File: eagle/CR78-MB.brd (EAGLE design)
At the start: 100 x 80 mm, 44 parts, among them IC1 40106N, Q510 2N3904, Q518 2N3904, Q526 2N3904, Q7 2N3904

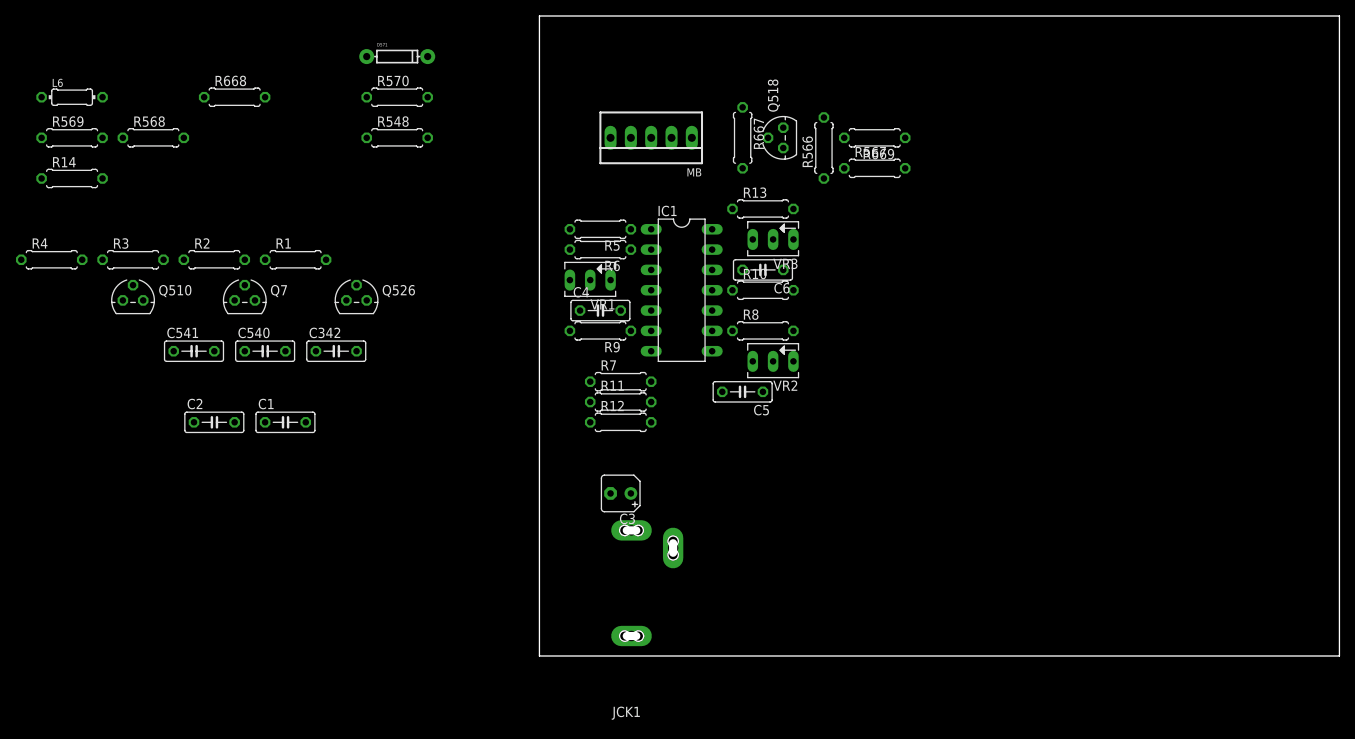
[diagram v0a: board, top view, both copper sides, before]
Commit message: parts on the brd
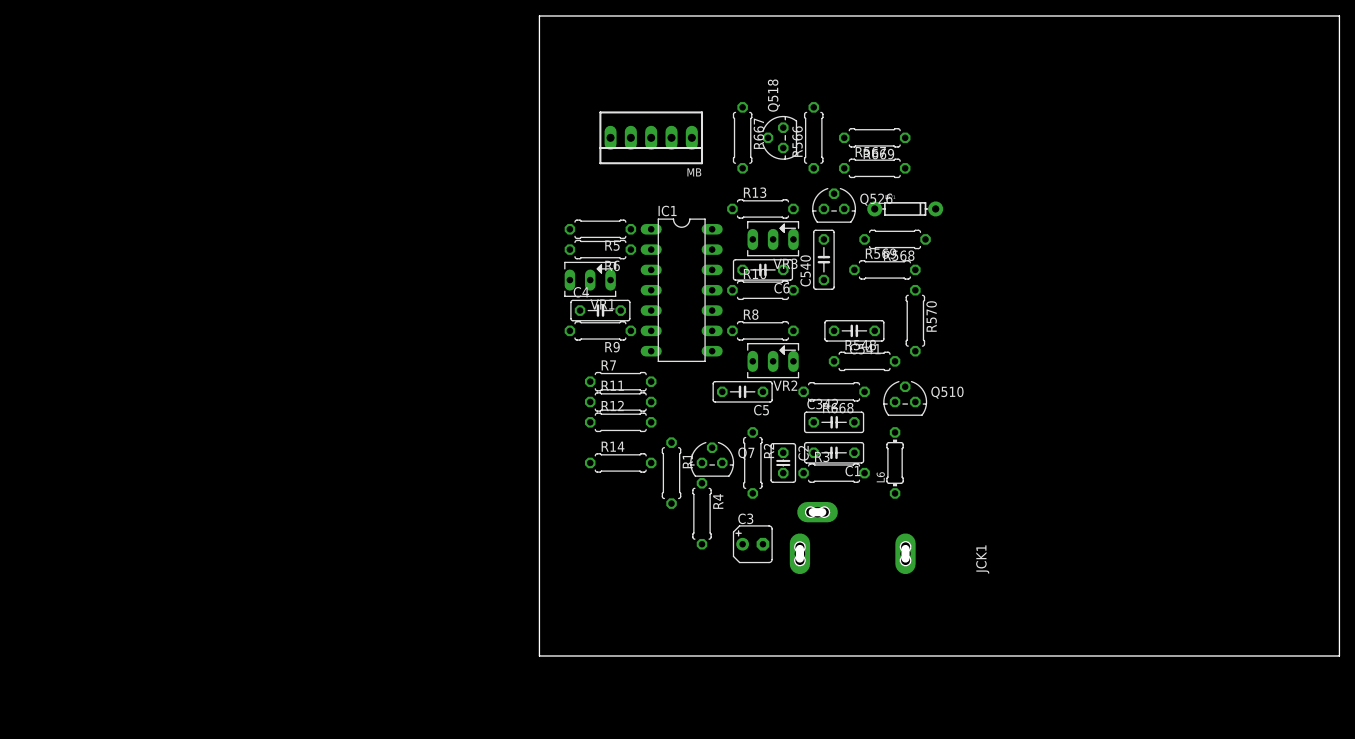
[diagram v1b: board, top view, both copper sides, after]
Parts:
- C2: device rcl:C050-025X075 -> rcl:C025-030X050
- moved L6 112.6 mm to (44.5, 24.1), turned to 90 degrees
- moved R569 102.9 mm to (43.2, 48.3)
- moved Q510 97.4 mm to (45.7, 31.8)
- moved R568 93.6 mm to (44.5, 52.1), turned to 180 degrees
- moved R3 91.6 mm to (36.8, 22.9)
- moved R4 87.3 mm to (20.3, 17.8), turned to 270 degrees
- moved R668 83.5 mm to (36.8, 33.0), turned to 180 degrees
- moved C541 82.6 mm to (39.4, 40.6), turned to 180 degrees
- moved R14 77.3 mm to (10.2, 24.1)
- moved R2 71.9 mm to (26.7, 24.1), turned to 270 degrees
- moved C2 71.3 mm to (30.5, 24.1), turned to 270 degrees
- moved C540 70.8 mm to (35.6, 49.5), turned to 90 degrees
- moved R570 70.5 mm to (47.0, 41.9), turned to 270 degrees
- moved C1 68.7 mm to (36.8, 25.4), turned to 180 degrees
- moved D571 66.3 mm to (45.7, 55.9)
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
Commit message: 96pct auto
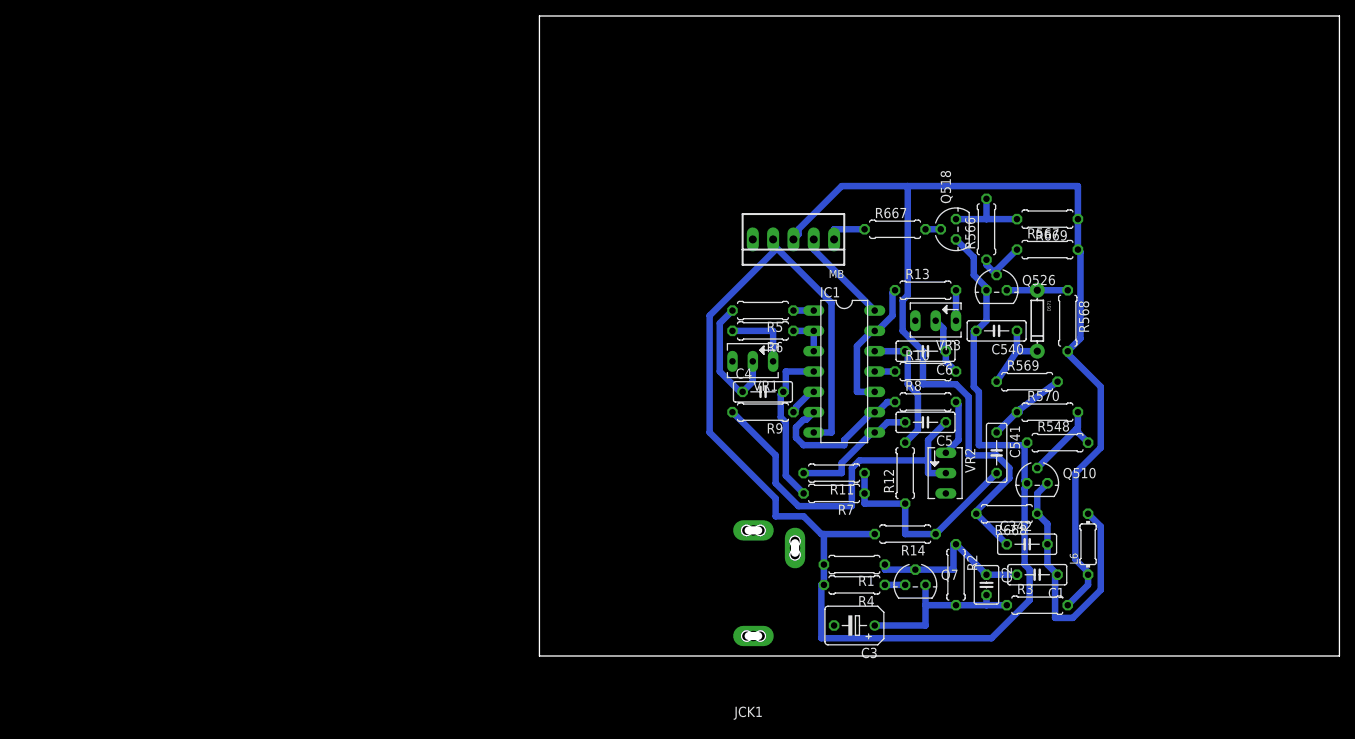
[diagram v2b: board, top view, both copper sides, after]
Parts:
- C3: device rcl:B45181A -> rcl:B45181B
- moved R14 36.7 mm to (45.7, 15.2), turned to 180 degrees
- moved R12 36.1 mm to (45.7, 22.9), turned to 90 degrees
- moved R3 30.3 mm to (62.2, 6.35)
- moved R7 30.1 mm to (36.8, 20.3), turned to 180 degrees
- moved C2 29.6 mm to (55.9, 8.89)
- moved Q7 29.6 mm to (47.0, 8.89)
- moved C1 29.6 mm to (62.2, 10.2)
- moved R2 29.0 mm to (52.1, 10.2)
- moved C342 28.5 mm to (61.0, 14.0)
- moved R11 28.1 mm to (36.8, 22.9), turned to 180 degrees
- moved R668 26.4 mm to (58.4, 17.8)
- moved L6 26.2 mm to (68.6, 14.0)
- moved R548 26.2 mm to (64.8, 26.7)
- moved VR2 25.7 mm to (50.8, 22.9), turned to 270 degrees
- moved R1 25.6 mm to (39.4, 11.4), turned to 180 degrees
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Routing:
- net GND: track 0.00 -> 180.0 mm
- net +12V: track 0.00 -> 154.9 mm
- net N$29: track 0.00 -> 46.0 mm
- net N$27: track 0.00 -> 36.1 mm
- net N$3: track 0.00 -> 27.3 mm
- net N$16: track 0.00 -> 22.9 mm
- net N$18: track 0.00 -> 22.1 mm
- net N$22: track 0.00 -> 20.4 mm
- net N$6: track 0.00 -> 19.7 mm
- net N$10: track 0.00 -> 17.3 mm
- net N$14: track 0.00 -> 16.7 mm
- net N$28: track 0.00 -> 16.5 mm
- net N$11: track 0.00 -> 16.1 mm
- net +5V: track 0.00 -> 12.0 mm
- net N$13: track 0.00 -> 11.4 mm
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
